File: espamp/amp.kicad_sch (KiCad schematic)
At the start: 37 parts, among them U501 TAS5825MRHB, U502 MPP684J2S1001, U503 MPP684J2S1001, U504 MPP684J2S1001, U505 MPP684J2S1001

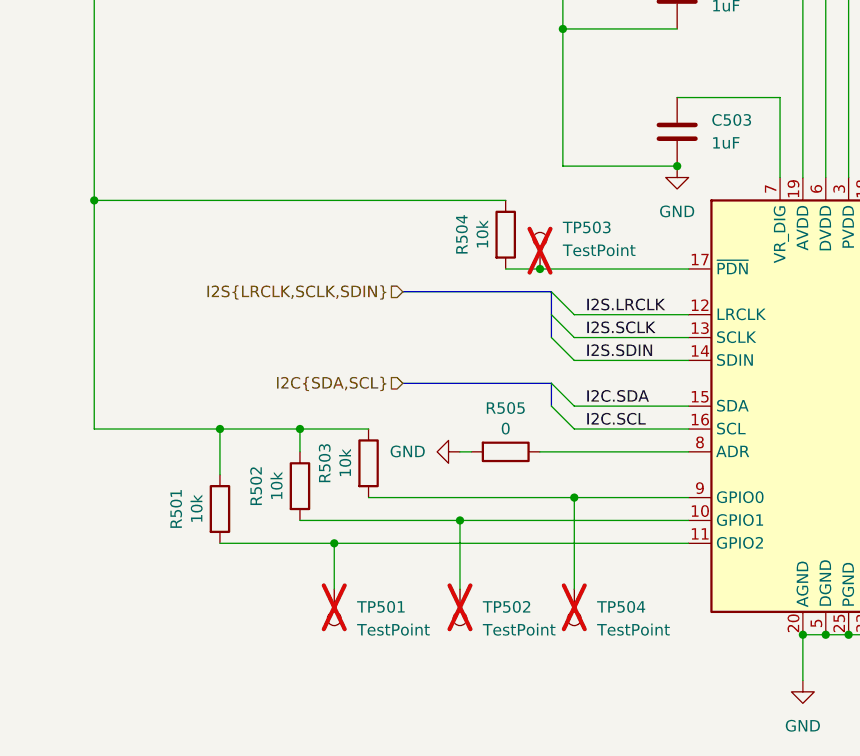
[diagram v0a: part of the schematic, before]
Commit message: espamp revisions
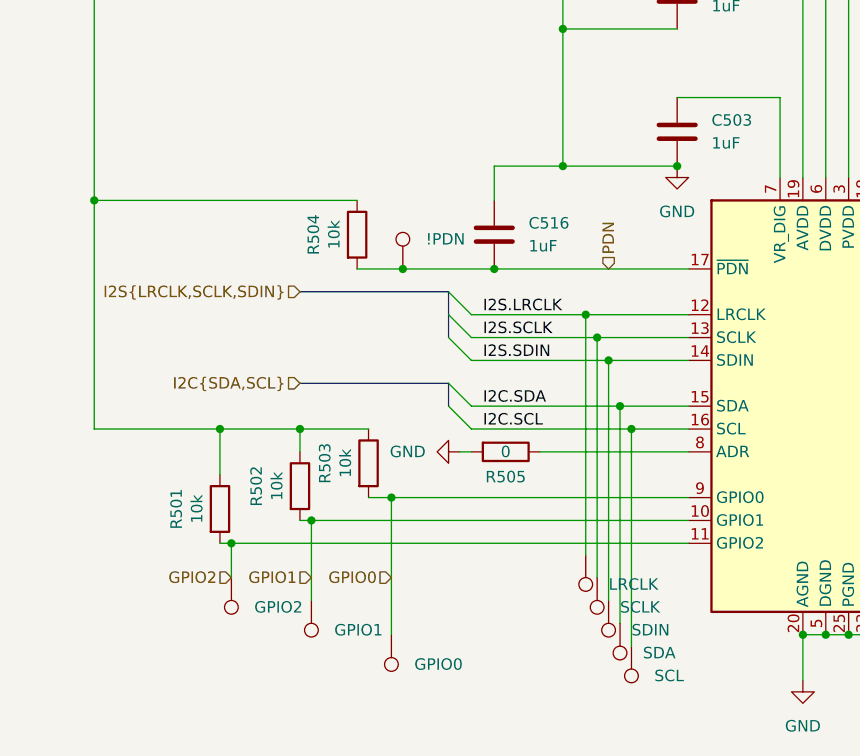
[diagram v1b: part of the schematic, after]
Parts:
- removed TP501, TP502, TP503, TP504: TestPoint, Connector_PinHeader_1.00mm:PinHeader_1x01_P1.00mm_Vertical, symbol Connector:TestPoint
- added C516: 1uF, Capacitor_SMD:C_0603_1608Metric, symbol Device:C
- added TP501, TP502, TP503, TP504, TP505, TP506, TP507, TP508, TP509: LabeledTestPoint, easyeda2kicad:LabeledTestPoint, symbol easyeda2kicad:LabeledTestPoint
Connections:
- net GND: now also C516.1
- net I2C.SCL: now also TP508.1
- net I2C.SDA: now also TP507.1
- net I2S.LRCLK: now also TP504.1
- net I2S.SCLK: now also TP505.1
- net I2S.SDIN: now also TP506.1
- net GPIO2: now reaches R501.2, U501.11 (GPIO2)
- net GPIO2: now also TP501.1
- net GPIO0: now reaches R503.2, U501.9 (GPIO0)
- net GPIO0: now also TP503.1
- net GPIO1: now reaches R502.2, U501.10 (GPIO1)
- net GPIO1: now also TP502.1
- net PDN: now reaches R504.2, U501.17 (~{PDN})
- net PDN: now also C516.2, TP509.1
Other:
- moved on the sheet: R504
